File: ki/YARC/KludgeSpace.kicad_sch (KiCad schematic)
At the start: 5 parts, among them J8 6-PIN FROM MCR, U100 74LS32, U101 74LS157, U139 74HC74, U140 74LS32

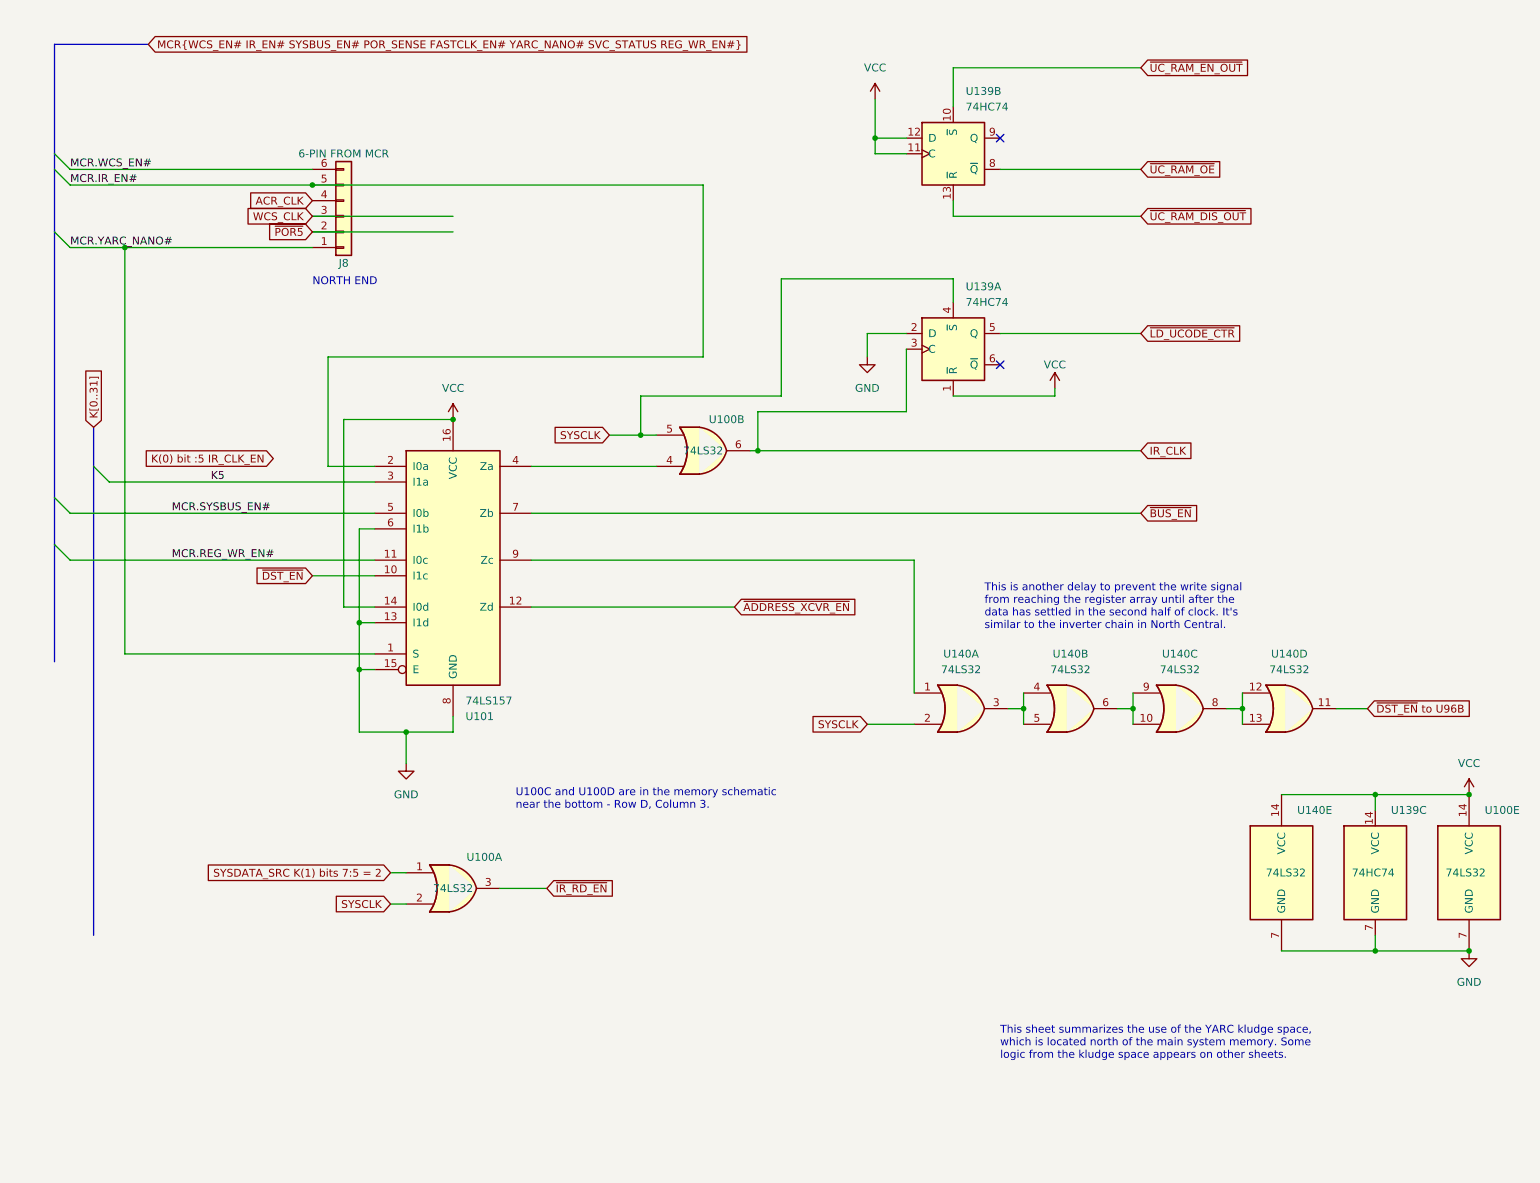
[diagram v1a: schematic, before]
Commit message: Ongoing schematic changes
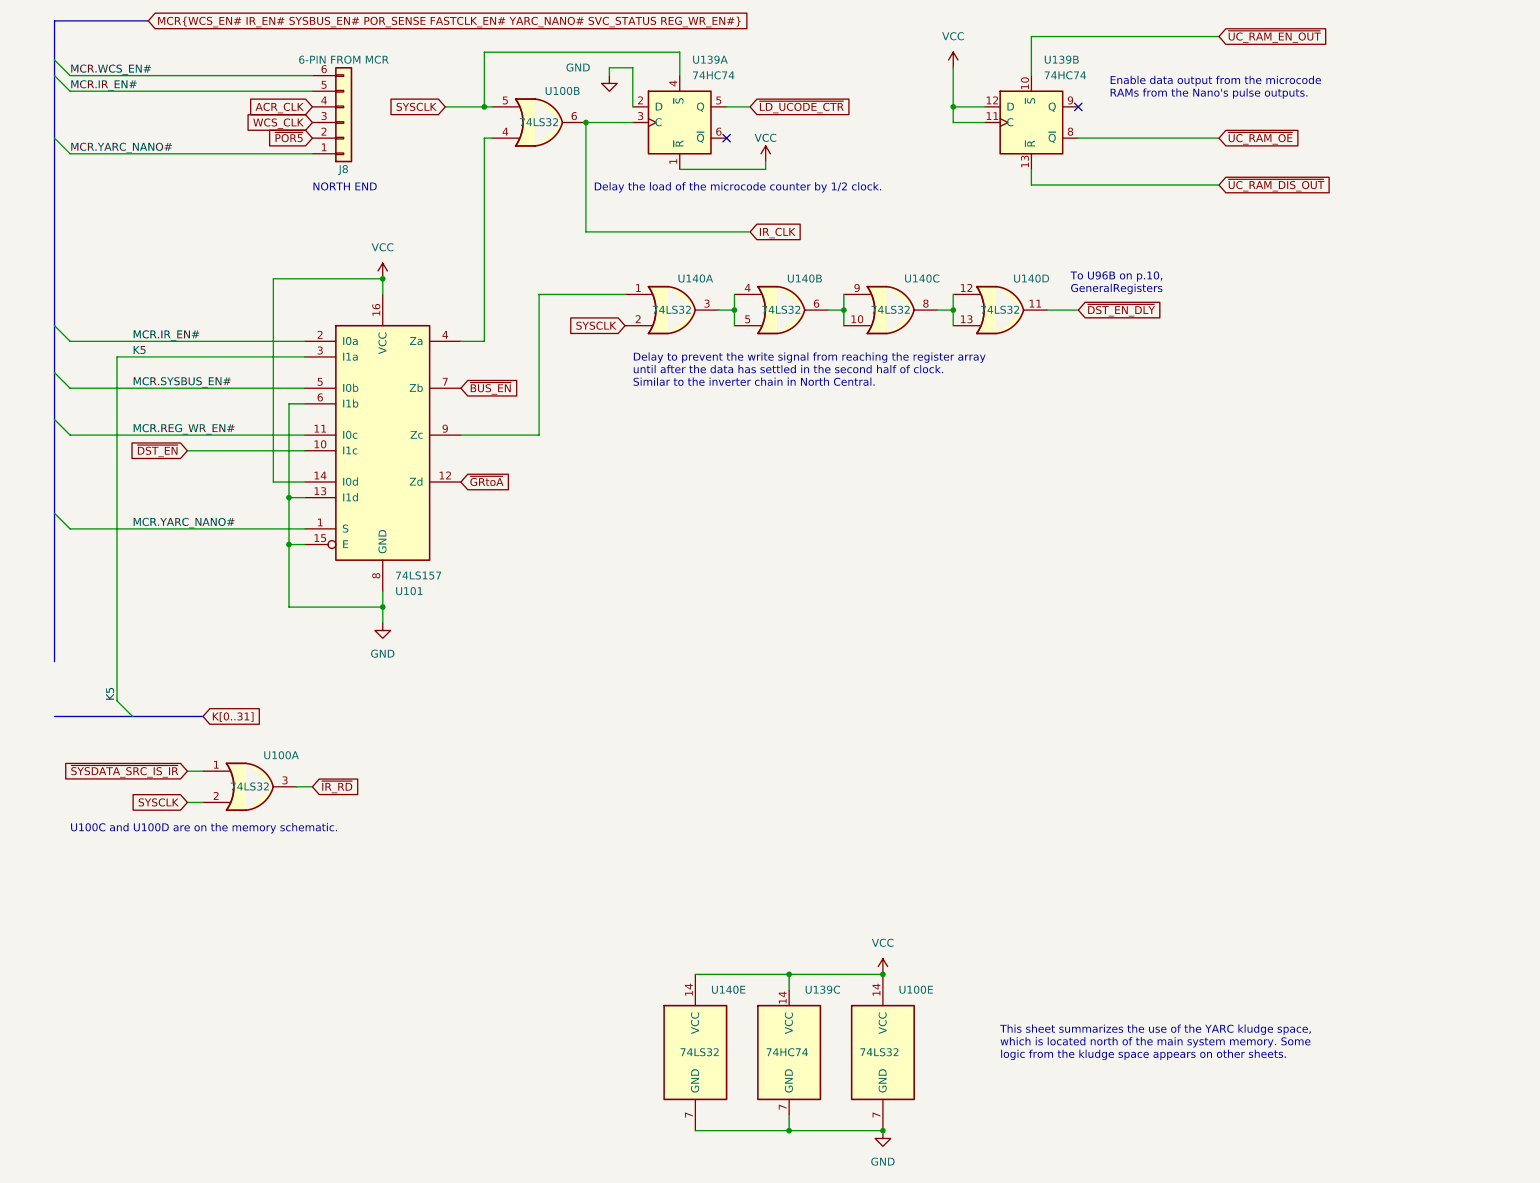
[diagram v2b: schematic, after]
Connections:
- net SYSDATA_SRC K(1) bits 7:5 = 2 renamed ~{SYSDATA_SRC_IS_IR}
- net ~{ADDRESS_XCVR_EN} renamed ~{GRtoA}
- net ~{DST_EN} to U96B renamed ~{DST_EN_DLY}
- net ~{IR_RD_EN} renamed ~{IR_RD}
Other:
- note added: "Delay the load of the microcode counter by 1/2 clock."
- note added: "Delay to prevent the write signal from reaching the register array until after the data has settled in the second half of clock. Similar to the inverter chain in North Central."
- note added: "Enable data output from the microcode RAMs from the Nano's pulse outputs."
- note added: "To U96B on p.10, GeneralRegisters"
- note added: "U100C and U100D are on the memory schematic."
- note removed: "This is another delay to prevent the write signal from reaching the register array until after the data has settled in the second half of clock. It's similar to the inverter chain in North Central."
- note removed: "U100C and U100D are in the memory schematic near the bottom - Row D, Column 3."
- moved on the sheet: J8, U100A, U100E, U101, U139A, U139B, U139C, U140A, U140B, U140C, U140D, U140E
